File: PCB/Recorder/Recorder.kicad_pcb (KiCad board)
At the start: 2 copper layers, 70 x 70 mm, 54 parts, among them J1 Battery, J2 Reset, J3 TC2030-USB-NL-DS, J4 TF_PUSH, J5 USB-C-Socket-H, Q2 CJ2301, SW1 SW_Push, U1 R, U2 L, U3 TP4054, U4 ME6211C33M5G-N, U5 MAX98357A, U6 ESP32-S3-MINI-1

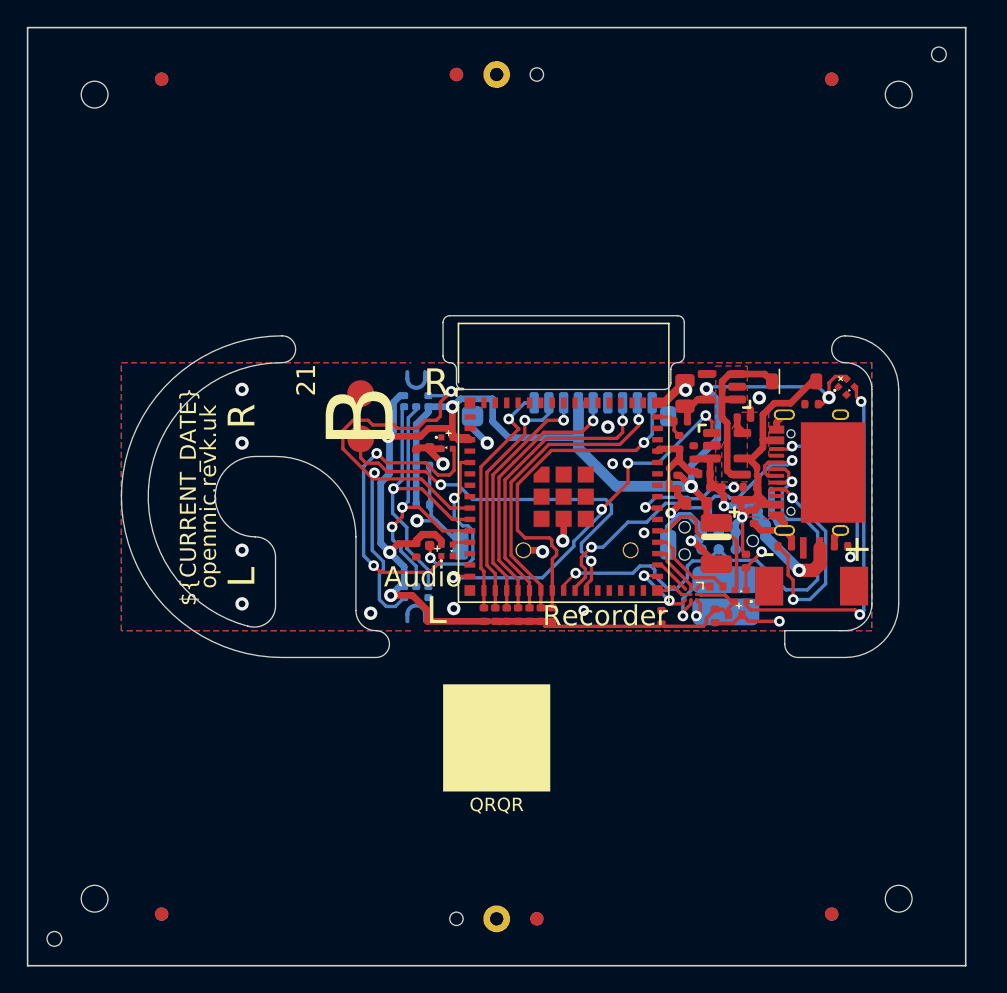
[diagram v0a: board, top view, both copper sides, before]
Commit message: Tidy
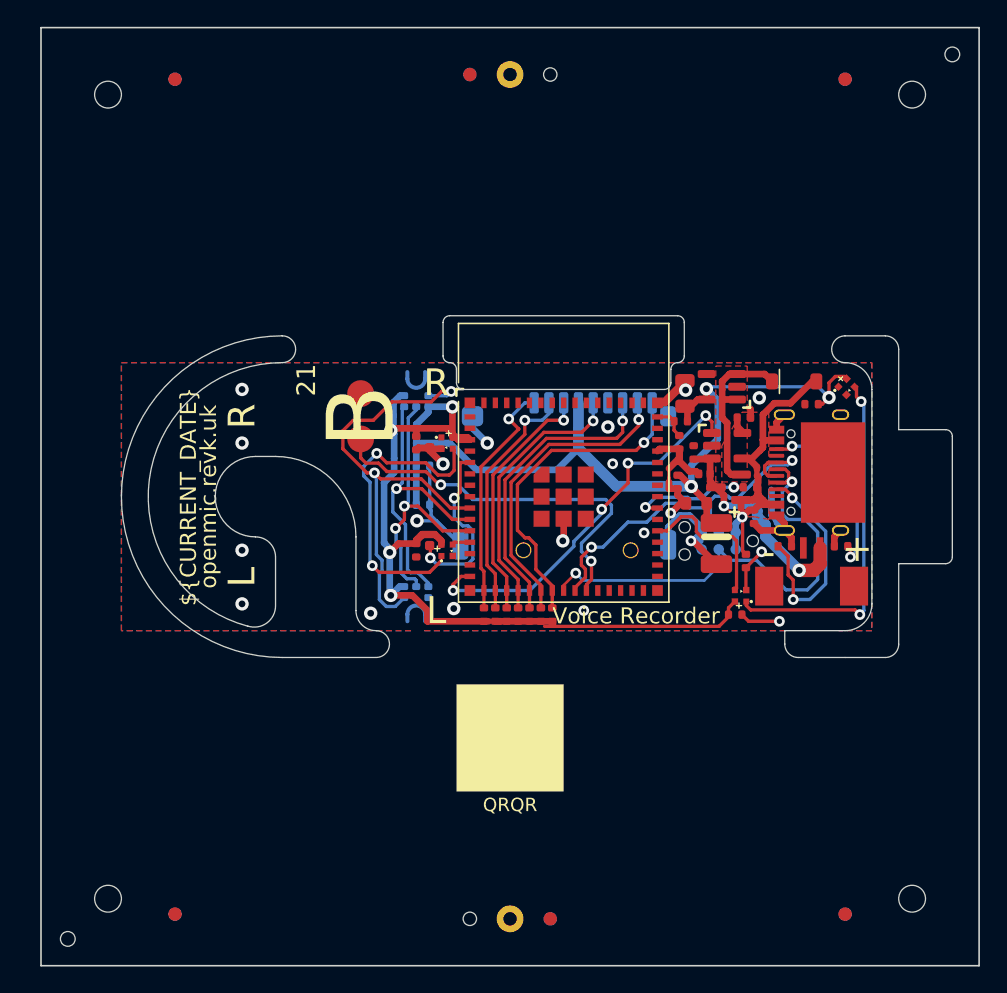
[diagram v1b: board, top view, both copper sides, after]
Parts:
- removed C12: 10uF, RevK:C_0402
- removed C14: 100nF, RevK:C_0402
- removed R4: 634K, RevK:R_0402
- removed TP1: +, RevK:SolderPadSmall
- removed TP2: -, RevK:SolderPadSmall
- removed U5: MAX98357A, RevK:WLP-1.437mmx1.347mm-0.21mm-ball
- moved V2 1.50 mm to (96.5, 110.0)
- moved PCB1 1.00 mm to (96.0, 100.0)
- moved V1 1.00 mm to (96.0, 90.0)
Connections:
- net SDMISO renamed SDDAT0
- net SDMOSI renamed SDCMD
- net SDSCK renamed SDCLK
- net SDSS renamed SDDAT3
- U6 pad 31: SKPWS -> unconnected-(U6-GPIO35-Pad31)
- U6 pad 32: SKPSCK -> unconnected-(U6-GPIO36-Pad32)
- U6 pad 33: SKPSD -> unconnected-(U6-GPIO37-Pad33)
- U6 pad 34: SKPPWR -> unconnected-(U6-GPIO38-Pad34)
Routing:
- net SKPPWR: track 6.62 -> 0.00 mm
- net GND: track 71.6 -> 65.1 mm, vias 21 -> 20
- net SKPWS: track 4.62 -> 0.00 mm, vias 2 -> 0
- net Net-(U5-OUTN): track 4.43 -> 0.00 mm, vias 1 -> 0
- net SKPSD: track 3.77 -> 0.00 mm
- net SKPSCK: track 2.42 -> 0.00 mm
- net +3V3: track 133.4 -> 131.6 mm
- net SCK: track 37.2 -> 35.9 mm
- net SDCD: track 25.6 -> 24.4 mm
- net CHARGING: track 27.9 -> 29.0 mm
- net Net-(U5-OUTP): track 1.02 -> 0.00 mm, vias 1 -> 0
- net D-: track 37.5 -> 36.4 mm
- net Net-(U5-~{SD_MODE}): track 0.60 -> 0.00 mm
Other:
- board text added: "1 8"
- board text added: "12 13 14 15 16 17 18"
- board text added: "41 18"
- board text added: "BTN LED"
- board text added: "Baking not required"
- board text added: "DAT2 DAT3 MOSI SCK DAT0 DAT1 CD"
- board text added: "VBUS CHRG"
- board text added: "Voice Recorder"
- board text removed: "1"
- board text removed: "12 13 14 15 17"
- board text removed: "18"
- board text removed: "35 36"
- board text removed: "37 38"
- board text removed: "41"
- board text removed: "8"
- board text removed: "A"
- board text removed: "Audio"
- board text removed: "B"
- board text removed: "BTN"
- board text removed: "Baking for D1 is not required"
- board text removed: "CHG"
- board text removed: "D P"
- board text removed: "Recorder"
- board text removed: "SPK"
- board text removed: "SS MOSI SCK MISO CD"
- board text removed: "VBUS"
- board text removed: "W C"
